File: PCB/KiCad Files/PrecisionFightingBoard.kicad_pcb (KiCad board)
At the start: 2 copper layers, 12 parts, among them J1 Conn_01x04_Male, J10 ST01x05, J2 Screw_Terminal_01x04, J6 Conn_02x10_Odd_Even, J7 ST01x05, J8 ST01x05, J9 ST01x05, U1 Teensy4.0

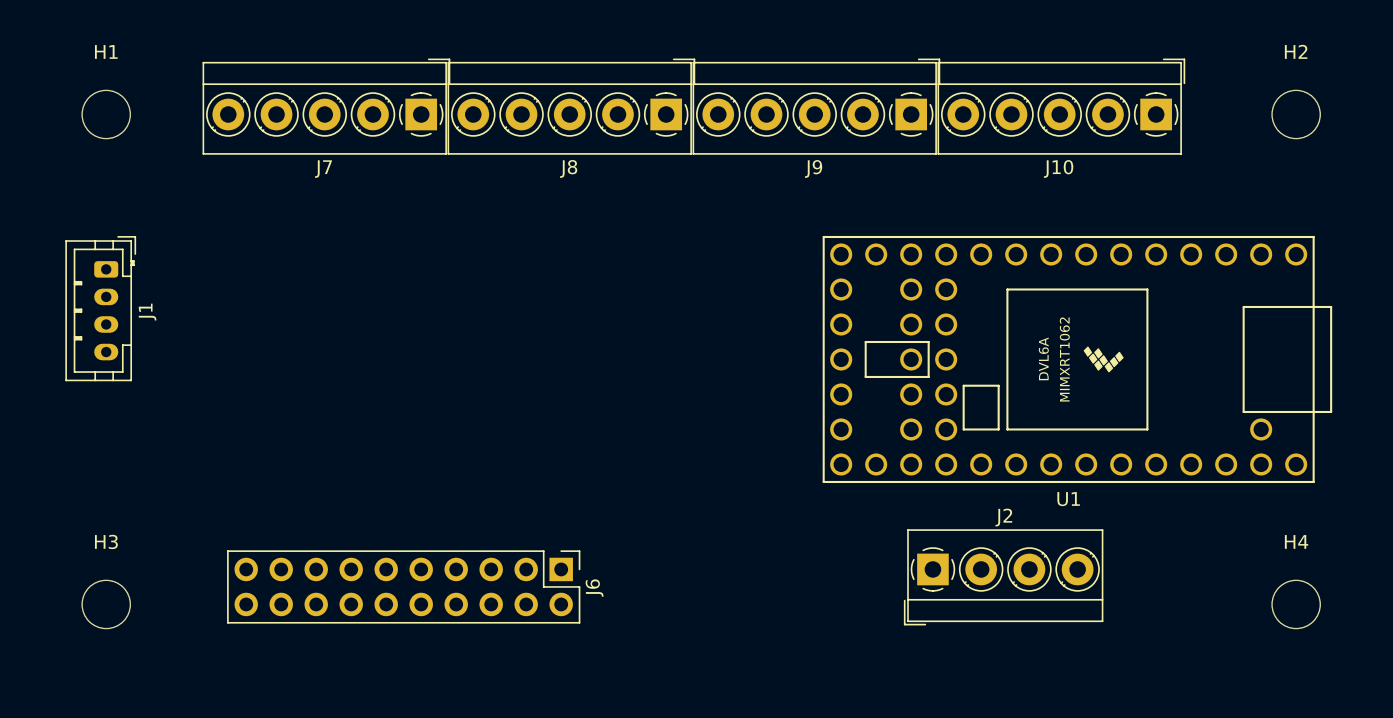
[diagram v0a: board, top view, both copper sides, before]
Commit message: Wired
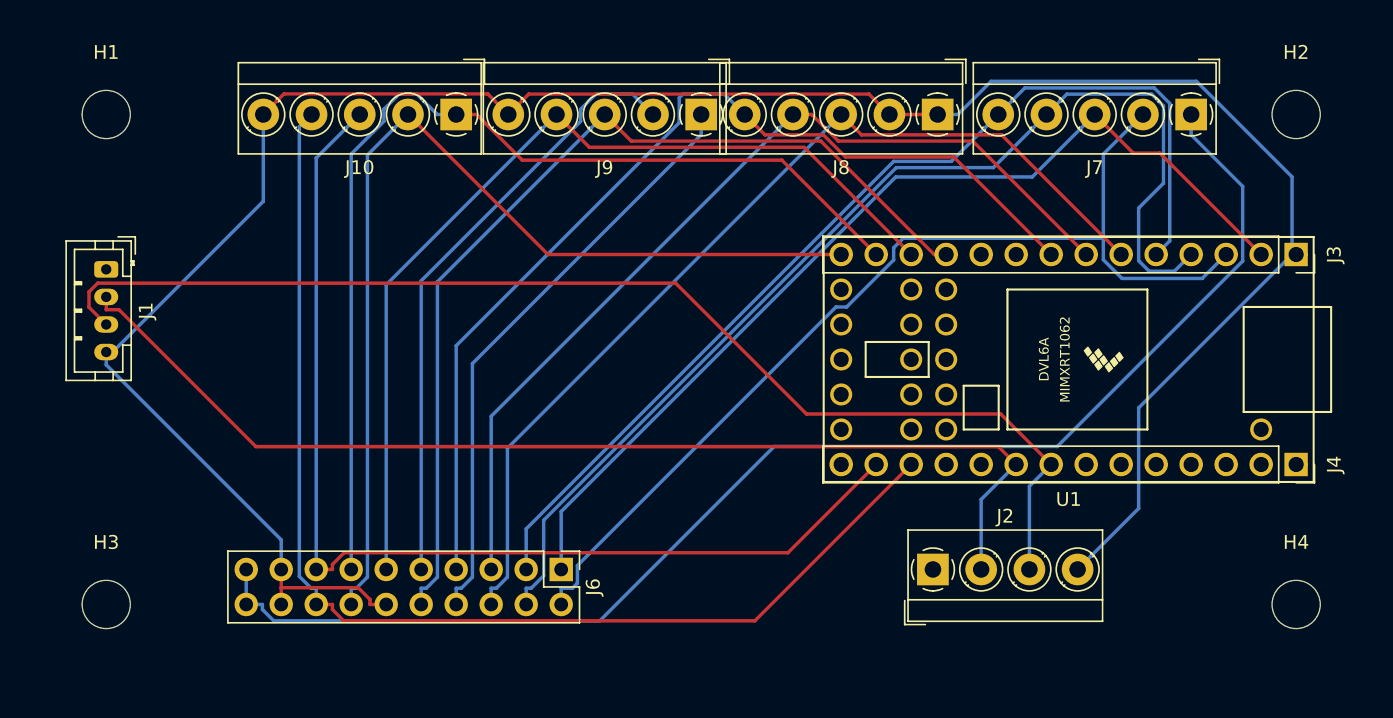
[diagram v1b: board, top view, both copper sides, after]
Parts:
- added J3: Conn_01x14_Socket, Connector_PinSocket_2.54mm:PinSocket_1x14_P2.54mm_Vertical, F.Cu at (160.0, 58.4)
- added J4: Conn_01x14_Socket, Connector_PinSocket_2.54mm:PinSocket_1x14_P2.54mm_Vertical, F.Cu at (160.0, 73.7)
- moved J7 55.9 mm to (152.4, 48.3)
- moved J10 50.8 mm to (99.1, 48.3)
- moved J8 19.7 mm to (134.0, 48.3)
- moved J9 15.2 mm to (116.8, 48.3)
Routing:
- net /GND: track 0.00 -> 170.6 mm
- net /5V: track 0.00 -> 98.6 mm
- net /R3: track 0.00 -> 86.7 mm
- net /LT: track 0.00 -> 85.2 mm
- net /LEFT: track 0.00 -> 81.6 mm
- net /L3: track 0.00 -> 80.3 mm
- net /RT: track 0.00 -> 78.3 mm
- net /A: track 0.00 -> 75.4 mm
- net /RIGHT: track 0.00 -> 74.7 mm
- net /DOWN: track 0.00 -> 74.2 mm
- net /B: track 0.00 -> 73.1 mm
- net /START: track 0.00 -> 72.9 mm
- net /UP: track 0.00 -> 71.2 mm
- net /HOME: track 0.00 -> 70.8 mm
- net /RB: track 0.00 -> 70.3 mm
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
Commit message: add gerber files
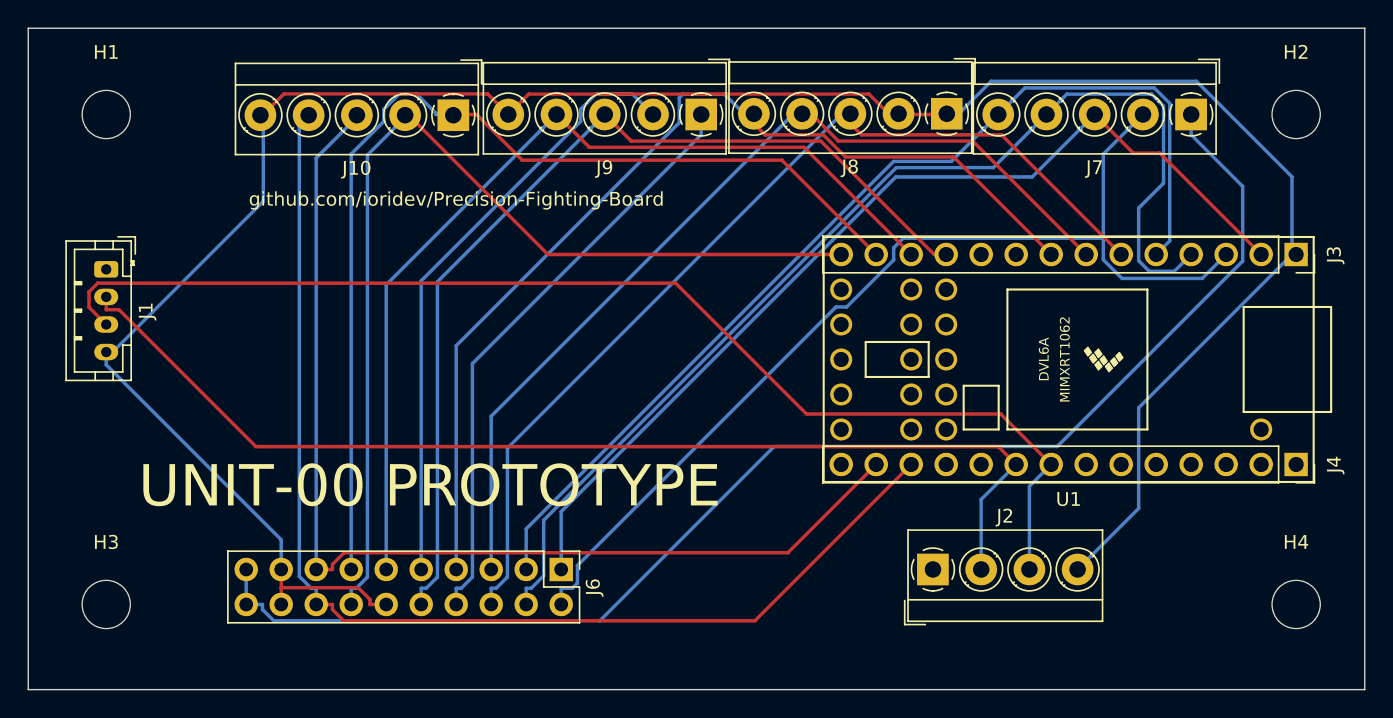
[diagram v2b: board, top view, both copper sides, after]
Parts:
- moved J8 0.67 mm to (134.7, 48.2)
- moved J10 0.21 mm to (98.9, 48.3)
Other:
- board outline added: 97 x 48 mm
- board text added: "UNIT-00 PROTOTYPE"
- board text added: "github.com/ioridev/Precision-Fighting-Board"
